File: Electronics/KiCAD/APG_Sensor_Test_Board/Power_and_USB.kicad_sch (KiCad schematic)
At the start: 12 parts, among them J4 USB_C_Receptacle_USB2.0_16P, U6 TLV1117-33

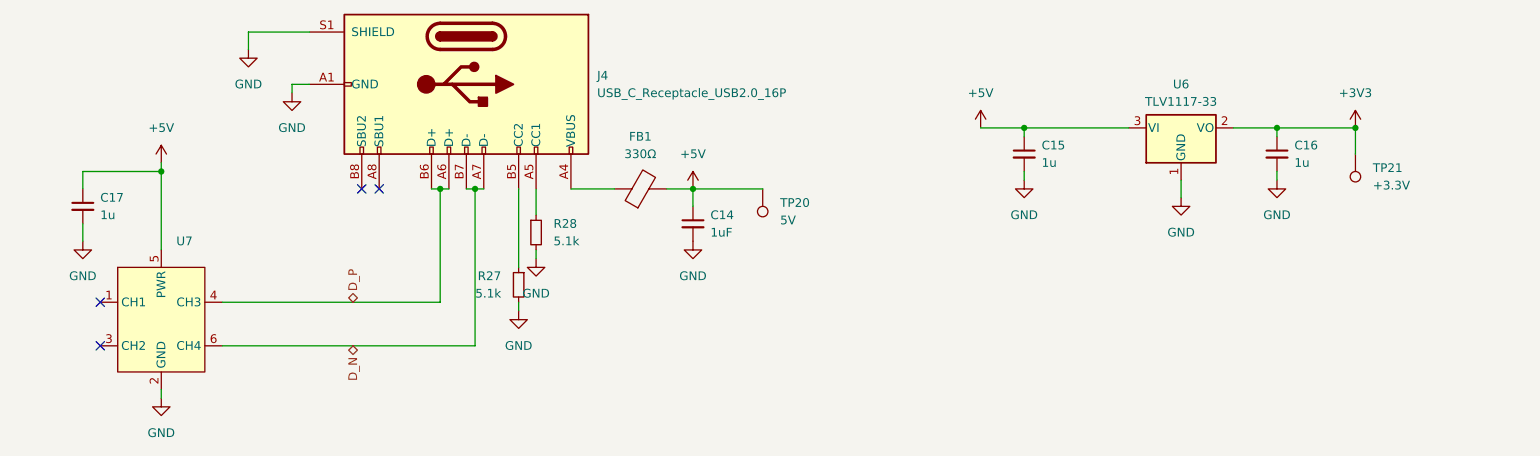
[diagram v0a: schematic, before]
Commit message: Layout and routing
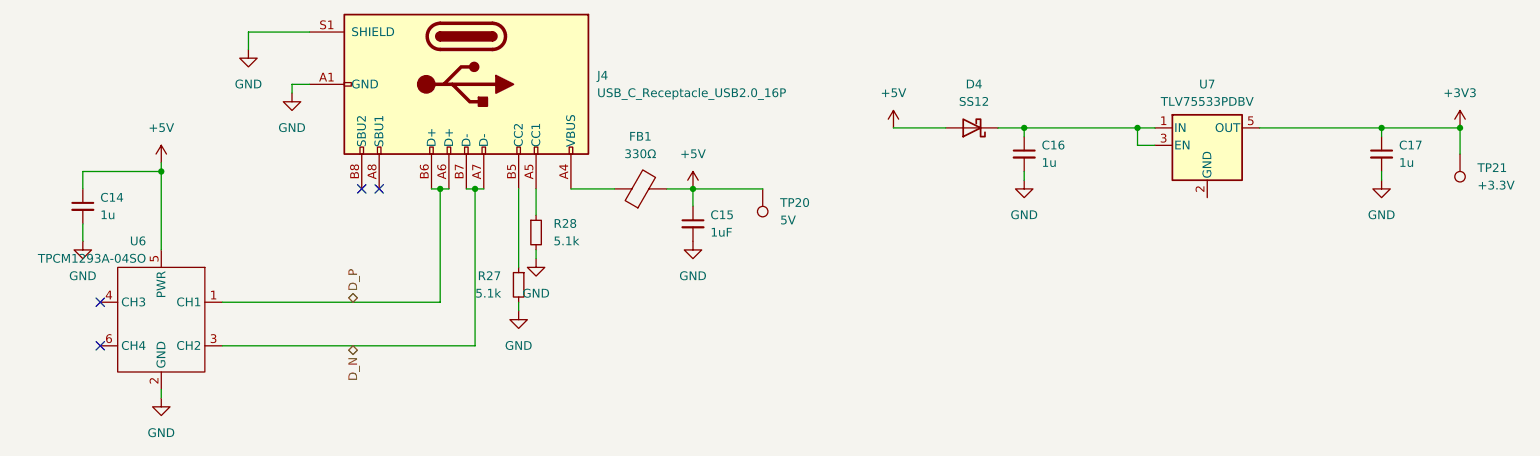
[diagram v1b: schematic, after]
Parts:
- removed U6: TLV1117-33, Package_TO_SOT_SMD:SOT-223-3_TabPin2, symbol Regulator_Linear:TLV1117-33
- added D4: SS12, Diode_SMD:D_SMA, symbol Device:D_Schottky
- added U7: TLV75533PDBV, Package_TO_SOT_SMD:SOT-23-5, symbol Regulator_Linear:TLV75533PDBV
- C14: renamed from C17; footprint Capacitor_SMD:C_0805_2012Metric -> Capacitor_SMD:C_0603_1608Metric
- C15: renamed from C14; footprint Capacitor_SMD:C_0805_2012Metric -> Capacitor_SMD:C_0603_1608Metric
- C16: renamed from C15; footprint Capacitor_SMD:C_0805_2012Metric -> Capacitor_SMD:C_0603_1608Metric
- C17: renamed from C16; footprint Capacitor_SMD:C_0805_2012Metric -> Capacitor_SMD:C_0603_1608Metric
- R27, R28: footprint Resistor_SMD:R_0805_2012Metric -> Resistor_SMD:R_0603_1608Metric
- TP20, TP21: footprint TestPoint:TestPoint_Pad_3.0x3.0mm -> TestPoint:TestPoint_Pad_D1.0mm
- U6: renamed from U7; value ~ -> TPCM1293A-04SO; footprint (none) -> Package_TO_SOT_SMD:SOT-23-6; JLCPCB (none) -> C558415
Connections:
- net +3V3: now also U7.5 (OUT)
- net +5V: now also D4.2 (A); no longer C16.1
- net D_N: now also U6.3 (CH2); no longer U6.6 (CH4)
- net D_P: now also U6.1 (CH1); no longer U6.4 (CH3)
- new net: C16.1, D4.1 (K), U7.1 (IN), U7.3 (EN)
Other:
- moved on the sheet: C17, TP21
